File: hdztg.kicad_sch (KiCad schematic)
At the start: 6 parts, among them J1 20374-R20E-31, J2 FPC-05FB-24PH20, Q1 BSS138DW-7-F

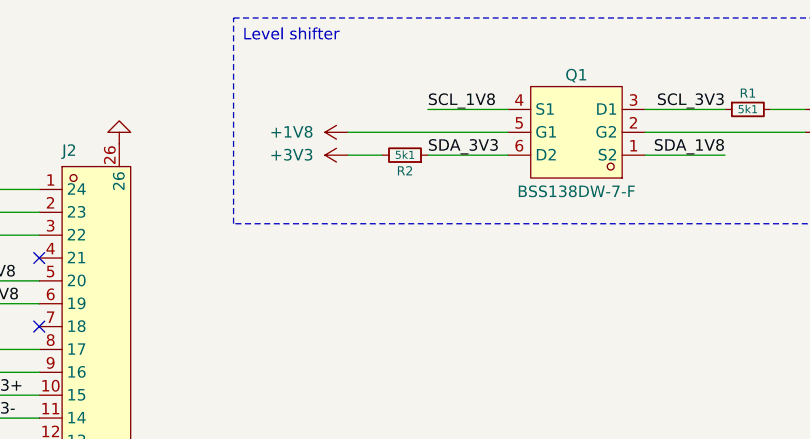
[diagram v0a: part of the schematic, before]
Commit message: jlcpcb production
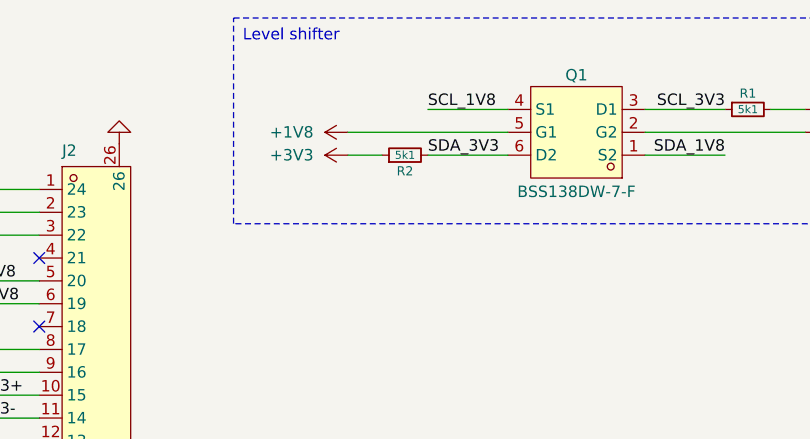
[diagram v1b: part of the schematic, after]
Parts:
- C1: footprint Capacitor_SMD:C_0201_0603Metric -> Capacitor_SMD:C_0402_1005Metric; Distributor Link https://lcsc.com/product-detail/Multilayer-Ceramic-Capacitors-MLCC-SMD-SMT_Samsung-Electro-Mechanics-CL03A105MO3NRNH_C307385.html -> https://lcsc.com/product-detail/Multilayer-Ceramic-Capacitors-MLCC-SMD-SMT_Samsung-Electro-Mechanics-CL05A105KO5NNNC_C29266.html?s_z=n_C29266; LCSC C307385 -> C29266; Manufacturer Part CL03A105MO3NRNH -> CL05A105KO5NNNC
- R1, R2: footprint Resistor_SMD:R_0201_0603Metric -> Resistor_SMD:R_0402_1005Metric; Distributor Link https://lcsc.com/product-detail/Chip-Resistor-Surface-Mount_YAGEO-RC0201FR-075K1L_C274341.html -> https://lcsc.com/product-detail/Chip-Resistor-Surface-Mount_UNI-ROYAL-0402WGF5101TCE_C25905.html; LCSC C274341 -> C25905; Manufacturer Part RC0201FR-075K1L -> 0402WGF5101TCE
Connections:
- net +3V3: now also R2.1; no longer R2.2
- net SDA_3V3: now also R2.2; no longer R2.1
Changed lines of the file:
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@@
 			)
 		)
-		(property "Footprint" "Resistor_SMD:R_0201_0603Metric"
+		(property "Footprint" "Resistor_SMD:R_0402_1005Metric"
 			(at 172.72 25.4 0)
 			(effects
@@
 			)
 		)
-		(property "Datasheet" "https://lcsc.com/datasheet/lcsc_datasheet_2506161045_YAGEO-RC0201FR-075K1L_C274341.pdf"
+		(property "Datasheet" "https://lcsc.com/datasheet/lcsc_datasheet_2411221127_UNI-ROYAL-0402WGF5101TCE_C25905.pdf"
 			(at 172.72 25.4 0)
 			(effects
@@
 			)
 		)
-		(property "Description" "Resistor, small symbol"
+		(property "Description" "62.5mW Thick Film Resistor 50V ±100ppm/℃ ±1% 5.1kΩ 0402 Chip Resistor - Surface Mount ROHS"
 			(at 172.72 25.4 0)
 			(effects
@@
 			)
 		)
-		(property "Manufacturer Part" "RC0201FR-075K1L"
+		(property "Manufacturer Part" "0402WGF5101TCE"
 			(at 172.72 25.4 90)
 			(effects
@@
 			)
 		)
-		(property "LCSC" "C274341"
+		(property "LCSC" "C25905"
 			(at 172.72 25.4 90)
 			(effects
@@
 			)
 		)
-		(property "Distributor Link" "https://lcsc.com/product-detail/Chip-Resistor-Surface-Mount_YAGEO-RC0201FR-075K1L_C274341.html"
+		(property "Distributor Link" "https://lcsc.com/product-detail/Chip-Resistor-Surface-Mount_UNI-ROYAL-0402WGF5101TCE_C25905.html"
 			(at 172.72 25.4 90)
 			(effects
@@
 	)
 	(symbol
+		(lib_id "Device:R_Small")
+		(at 134.62 30.48 90)
+		(unit 1)
+		(exclude_from_sim no)
+		(in_bom yes)
+		(on_board yes)
+		(dnp no)
+		(property "Reference" "R2"
+			(at 134.62 32.258 90)
+			(effects
+				(font
+					(size 1.016 1.016)
+				)
+			)
+		)
+		(property "Value" "5k1"
+			(at 134.62 30.48 90)
+			(effects
+				(font
+					(size 0.889 0.889)
+				)
+			)
+		)
+		(property "Footprint" "Resistor_SMD:R_0402_1005Metric"
+			(at 134.62 30.48 0)
+			(effects
+				(font
+					(size 1.27 1.27)
+				)
+				(hide yes)
+			)
+		)
+		(property "Datasheet" "https://lcsc.com/datasheet/lcsc_datasheet_2411221127_UNI-ROYAL-0402WGF5101TCE_C25905.pdf"
+			(at 134.62 30.48 0)
+			(effects
+				(font
+					(size 1.27 1.27)
+				)
+				(hide yes)
+			)
+		)
+		(property "Description" "62.5mW Thick Film Resistor 50V ±100ppm/℃ ±1% 5.1kΩ 0402 Chip Resistor - Surface Mount ROHS"
+			(at 134.62 30.48 0)
+			(effects
+				(font
+					(size 1.27 1.27)
+				)
+				(hide yes)
+			)
+		)
+		(property "Manufacturer Part" "0402WGF5101TCE"
+			(at 134.62 30.48 90)
+			(effects
+				(font
+					(size 1.27 1.27)
+				)
+				(hide yes)
+			)
+		)
+		(property "LCSC" "C25905"
+			(at 134.62 30.48 90)
+			(effects
+				(font
+					(size 1.27 1.27)
+				)
+				(hide yes)
+			)
+		)
+		(property "Distributor Link" "https://lcsc.com/product-detail/Chip-Resistor-Surface-Mount_UNI-ROYAL-0402WGF5101TCE_C25905.html"
+			(at 134.62 30.48 90)
+			(effects
+				(font
+					(size 1.27 1.27)
+				)
+				(hide yes)
+			)
+		)
+		(pin "1"
+		)
+		(pin "2"
+		)
+		(instances
+			(project "hdztg"
+				(path "/5fa3be86-0836-40c5-8497-58cbc35ea59a"
+					(reference "R2")
+					(unit 1)
+				)
+			)
+		)
+	)
+	(symbol
 		(lib_id "power:GND")
 		(at 102.87 97.79 0)
@@
 	)
 	(symbol
-		(lib_id "Device:R_Small")
-		(at 134.62 30.48 270)
-		(mirror x)
-		(unit 1)
-		(exclude_from_sim no)
-		(in_bom yes)
-		(on_board yes)
-		(dnp no)
-		(property "Reference" "R2"
-			(at 134.62 32.258 90)
-			(effects
-				(font
-					(size 1.016 1.016)
-				)
-			)
-		)
-		(property "Value" "5k1"
-			(at 134.62 30.48 90)
-			(effects
-				(font
-					(size 0.889 0.889)
-				)
-			)
-		)
-		(property "Footprint" "Resistor_SMD:R_0201_0603Metric"
-			(at 134.62 30.48 0)
-			(effects
-				(font
-					(size 1.27 1.27)
-				)
-				(hide yes)
-			)
-		)
-		(property "Datasheet" "https://lcsc.com/datasheet/lcsc_datasheet_2506161045_YAGEO-RC0201FR-075K1L_C274341.pdf"
-			(at 134.62 30.48 0)
-			(effects
-				(font
-					(size 1.27 1.27)
-				)
-				(hide yes)
-			)
-		)
-		(property "Description" "Resistor, small symbol"
-			(at 134.62 30.48 0)
-			(effects
-				(font
-					(size 1.27 1.27)
-				)
-				(hide yes)
-			)
-		)
-		(property "Manufacturer Part" "RC0201FR-075K1L"
-			(at 134.62 30.48 90)
-			(effects
-				(font
-					(size 1.27 1.27)
-				)
-				(hide yes)
-			)
-		)
-		(property "LCSC" "C274341"
-			(at 134.62 30.48 90)
-			(effects
-				(font
-					(size 1.27 1.27)
-				)
-				(hide yes)
-			)
-		)
-		(property "Distributor Link" "https://lcsc.com/product-detail/Chip-Resistor-Surface-Mount_YAGEO-RC0201FR-075K1L_C274341.html"
-			(at 134.62 30.48 90)
-			(effects
-				(font
-					(size 1.27 1.27)
-				)
-				(hide yes)
-			)
-		)
-		(pin "1"
-		)
-		(pin "2"
-		)
-		(instances
-			(project "hdztg"
-				(path "/5fa3be86-0836-40c5-8497-58cbc35ea59a"
-					(reference "R2")
-					(unit 1)
-				)
-			)
-		)
-	)
-	(symbol
 		(lib_id "power:GND")
 		(at 52.07 57.15 90)
@@
 			)
 		)
-		(property "Footprint" "Capacitor_SMD:C_0201_0603Metric"
+		(property "Footprint" "Capacitor_SMD:C_0402_1005Metric"
 			(at 45.72 87.63 0)
 			(effects
@@
 			)
 		)
-		(property "Description" "Unpolarized capacitor, small symbol"
+		(property "Description" "16V 1uF X5R ±10% 0402 Multilayer Ceramic Capacitors MLCC - SMD/SMT ROHS"
 			(at 45.72 87.63 0)
 			(effects
@@
 			)
 		)
-		(property "Manufacturer Part" "CL03A105MO3NRNH"
+		(property "Manufacturer Part" "CL05A105KO5NNNC"
 			(at 45.72 87.63 0)
 			(effects
@@
 			)
 		)
-		(property "LCSC" "C307385"
+		(property "LCSC" "C29266"
 			(at 45.72 87.63 0)
 			(effects
@@
 			)
 		)
-		(property "Distributor Link" "https://lcsc.com/product-detail/Multilayer-Ceramic-Capacitors-MLCC-SMD-SMT_Samsung-Electro-Mechanics-CL03A105MO3NRNH_C307385.html"
+		(property "Distributor Link" "https://lcsc.com/product-detail/Multilayer-Ceramic-Capacitors-MLCC-SMD-SMT_Samsung-Electro-Mechanics-CL05A105KO5NNNC_C29266.html?s_z=n_C29266"
 			(at 45.72 87.63 0)
 			(effects
